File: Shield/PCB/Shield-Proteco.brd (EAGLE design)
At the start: 100 x 80 mm, 28 parts

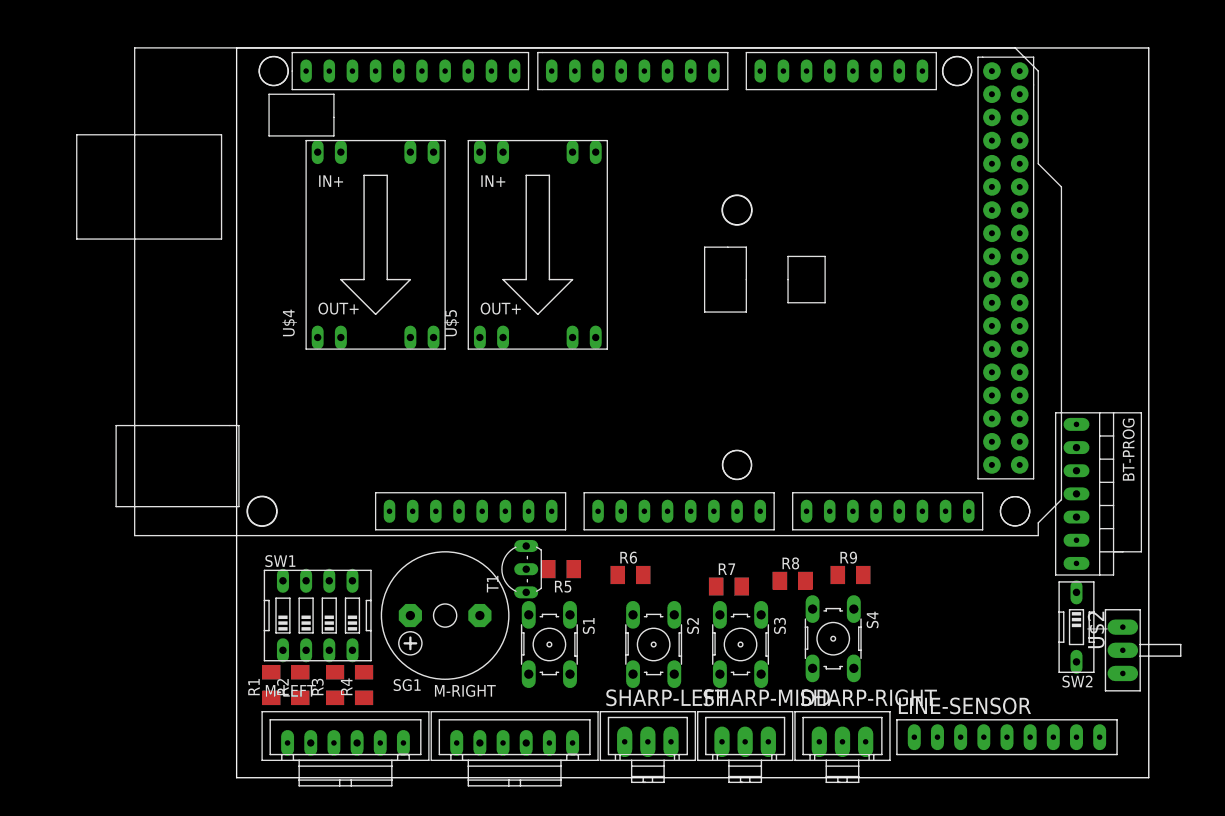
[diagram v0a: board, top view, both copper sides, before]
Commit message: Avance shield y correccion librerias
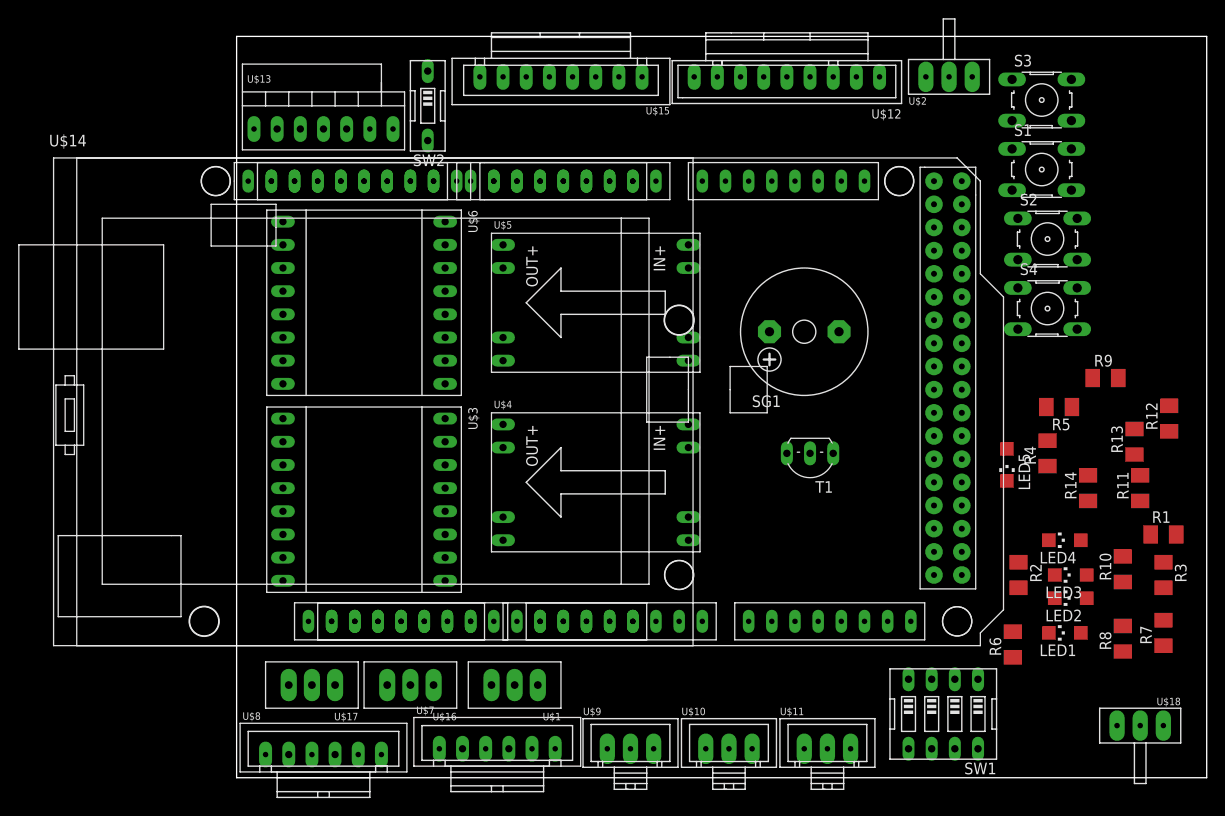
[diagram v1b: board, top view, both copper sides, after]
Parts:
- removed BT-PROG: HC-05-PROG, hc-xx:HC-05-PROG
- removed LINE-SENSOR: CNY70-ARRAY, Sensores:CNY70-ARRAY
- removed M-LEFT, M-RIGHT: POLOLU-MICROMOTOR, Motores:JST
- removed SHARP-LEFT, SHARP-MIDD, SHARP-RIGHT: SHARP, Sensores:SHARP
- added ARDUINO-MEGA: ARDUINO_MEGA, Arduino:ARDUINO-MEGA
- added LED1, LED2, LED3, LED4, LED5: (no value), led:CHIPLED_1206
- added R10, R11, R12, R13, R14: (no value), rcl:M1206
- added U$10, U$11, U$9: SHARP, Sensores:SHARP
- added U$12: CNY70-ARRAY, Sensores:CNY70-ARRAY
- added U$13: HC-05-PROG, hc-xx:HC-05-PROG
- added U$14: TFT_ARDUINO-UNO-MEGA, TFT:TFT-ARDUINO-UNO-MEGA
- added U$15: ACELEROMETER-MPU6050-JST, Sensores:ACELEROMETER-MPU6050-JST
- added U$16, U$17: SERVOMOTORES, Motores:SERVO
- added U$18: SLIDE-3, Interruptores:SLIDE-3
- added U$3, U$6: TB6612FNG, Driver-Motor:TB6612FNG
- added U$7, U$8: POLOLU-MICROMOTOR, Motores:JST
- U$1: value ARDUINO_MEGA -> SERVOMOTORES; device Arduino:ARDUINO-MEGA -> Motores:SERVO
- moved R1 99.2 mm to (101.6, 26.7), turned to 0 degrees
- moved R3 91.6 mm to (101.6, 22.2), turned to 270 degrees
- moved SW2 91.2 mm to (21.0, 73.7)
- moved R2 79.7 mm to (85.7, 22.2), turned to 270 degrees
- moved R4 79.1 mm to (88.9, 35.6)
- moved S1 75.0 mm to (88.3, 66.7), turned to 0 degrees
- moved SW1 69.4 mm to (77.5, 6.99), turned to 180 degrees
- moved S3 68.2 mm to (88.3, 74.3), turned to 0 degrees
- moved U$2 65.7 mm to (78.1, 76.8), turned to 0 degrees
- moved S2 62.0 mm to (88.9, 59.1), turned to 0 degrees
- moved R5 57.4 mm to (90.2, 40.6)
- moved SG1 50.2 mm to (62.2, 48.9)
- moved R7 47.9 mm to (101.6, 15.9), turned to 90 degrees
- moved S4 43.2 mm to (88.9, 51.4), turned to 0 degrees
- moved R6 42.6 mm to (85.1, 14.6), turned to 90 degrees
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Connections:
- new net N$17: U$15.SCL
- new net N$18: U$15.SDA
- new net N$19: U$15.XDA
- new net N$20: U$15.XCL
- new net N$21: U$15.ADO
- new net N$22: U$15.INT
- new net N$23: LED1.C, R10.2
- new net N$24: LED2.C, R11.2
- new net N$25: LED3.C, R12.2
- new net N$26: LED4.C, R13.2
- new net N$27: U$14.0-RX0
- new net N$28: U$14.3V3
- new net N$29: U$14.5V_1, U$18.P2
- new net N$30: U$14.GND_2
- new net N$31: U$14.GND_1
- new net N$32: U$14.VIN
- new net N$33: U$14.A0
- new net N$34: U$14.A1
- new net N$35: U$14.A2
- new net N$36: U$14.A3
- new net N$37: U$14.A4
- new net N$38: U$14.A5
- new net N$39: ARDUINO-MEGA.3V3
- new net N$40: ARDUINO-MEGA.5V_1
- new net N$41: ARDUINO-MEGA.GND_2
- new net N$42: ARDUINO-MEGA.GND_1
- new net N$43: ARDUINO-MEGA.VIN
- new net N$44: ARDUINO-MEGA.A0
- new net N$45: ARDUINO-MEGA.A1
- new net N$46: ARDUINO-MEGA.A2
- new net N$47: ARDUINO-MEGA.A3
- new net N$48: ARDUINO-MEGA.A4
- new net N$49: ARDUINO-MEGA.A5
- new net N$50: ARDUINO-MEGA.A6
- new net N$51: ARDUINO-MEGA.A7
- new net N$52: ARDUINO-MEGA.A8
- new net N$53: ARDUINO-MEGA.A9
- new net N$54: ARDUINO-MEGA.A10
- new net N$55: ARDUINO-MEGA.A11
- new net N$56: ARDUINO-MEGA.A12
- new net N$57: ARDUINO-MEGA.A13
- new net N$58: ARDUINO-MEGA.A14
- new net N$59: ARDUINO-MEGA.A15
- new net N$60: U$14.1-TX0
- new net N$61: U$14.2
- new net N$62: U$14.3
- new net N$63: U$14.4
- new net N$64: U$14.5
- new net N$65: U$14.6
- new net N$66: U$14.7
- new net N$67: U$14.AREF
- new net N$68: U$14.GND
- new net N$70: U$14.12
- new net N$71: U$14.11
- new net N$72: U$14.10
- new net N$73: U$14.9
- new net N$74: U$14.8
- new net N$75: U$1.SIGNAL
- new net N$76: U$16.SIGNAL
- new net N$77: U$17.SIGNAL
- new net N$78: ARDUINO-MEGA.SCL
- new net N$79: ARDUINO-MEGA.SDA
- new net N$80: ARDUINO-MEGA.AREF
- new net N$81: ARDUINO-MEGA.GND
- new net SD_SCK: ARDUINO-MEGA.13, U$14.13
- net 6V-DC-3A: now also U$3.VM, U$6.VM; no longer M-LEFT.VCC, M-RIGHT.VCC
- net GND: now also R10.1, R11.1, R12.1, R13.1, R14.1, U$1.GND, U$10.GND, U$11.GND, U$12.GND, U$13.GND, U$15.GND, U$16.GND, U$17.GND, U$3.GND, U$3.GND_1, U$3.GND_2, U$6.GND, U$6.GND_1, U$6.GND_2, U$7.GND, U$8.GND, U$9.GND; no longer BT-PROG.GND, LINE-SENSOR.GND, M-LEFT.GND, M-RIGHT.GND, SHARP-LEFT.GND, SHARP-MIDD.GND, SHARP-RIGHT.GND
- net N$16: now also U$13.RESET; no longer BT-PROG.RESET
- net N$7: now also U$9.DIST; no longer SHARP-LEFT.DIST
- net N$8: now also U$10.DIST; no longer SHARP-MIDD.DIST
- net N$9: now also U$11.DIST; no longer SHARP-RIGHT.DIST
- net RESET: now also ARDUINO-MEGA.RESET, U$14.RESET
- net RX0: now also U$13.RXD; no longer BT-PROG.RXD
- net SCD: now also U$12.SCD; no longer LINE-SENSOR.SCD
- net SCI: now also U$12.SCI; no longer LINE-SENSOR.SCI
- net SF: now also U$12.SF; no longer LINE-SENSOR.SF
- net SID: now also U$12.SID; no longer LINE-SENSOR.SID
- net SII: now also U$12.SII; no longer LINE-SENSOR.SII
- net SSD: now also U$12.SSD; no longer LINE-SENSOR.SSD
- net SSI: now also U$12.SSI; no longer LINE-SENSOR.SSI
- net TX0: now also U$13.TXD; no longer BT-PROG.TXD
- net VCC: now also U$1.VCC, U$10.VCC, U$11.VCC, U$12.VCC, U$13.VCC, U$15.VCC, U$16.VCC, U$17.VCC, U$18.COM, U$3.VCC, U$6.VCC, U$7.VCC, U$8.VCC, U$9.VCC; no longer BT-PROG.VCC, LINE-SENSOR.VCC, SHARP-LEFT.VCC, SHARP-MIDD.VCC, SHARP-RIGHT.VCC
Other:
- board size 100 x 80 mm -> 106.3 x 81.3 mm
